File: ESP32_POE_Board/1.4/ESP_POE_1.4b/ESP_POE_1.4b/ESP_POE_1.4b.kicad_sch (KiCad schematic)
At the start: 74 parts, among them J26 USB_C_Receptacle, J5 20021311-00012T4LF, J7 20021311-00012T4LF, Q1 Q12MHz/20pF/10ppm/4P/3.2x2.5mm, Q2 BC817-40(SOT23), Q3 BC817-40(SOT23), SW1 PTS815 SJM 250 SMTR LFS, U1 CH340T(SSOP20W), U3 BL4054B-42TPRN(SOT23-5), U6 ESP32-WROVER-E, U7 SY8089AAAC(SOT23-5), U8 SN74LVC1G04DBVR(SOT23-5)

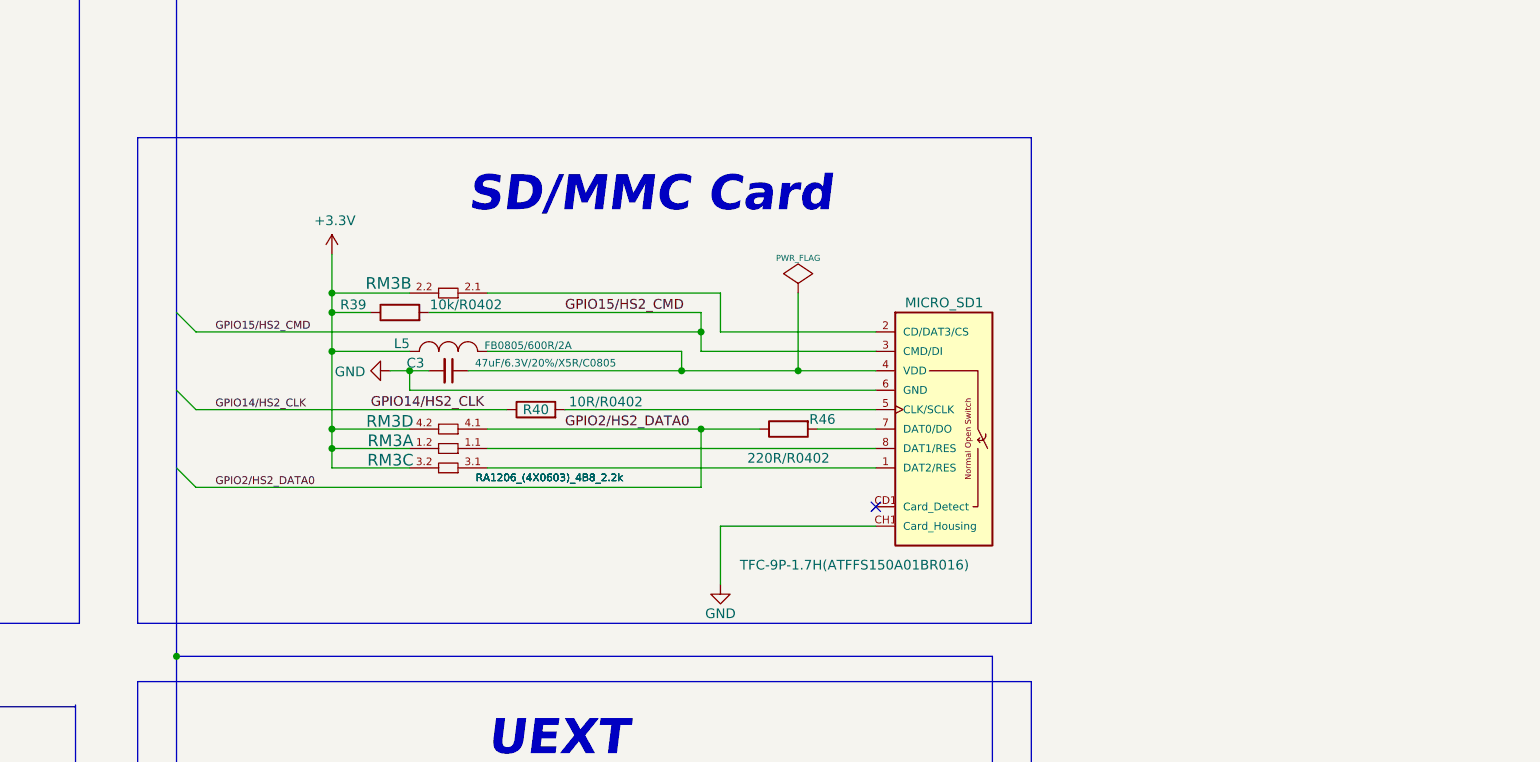
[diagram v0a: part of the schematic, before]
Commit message: fixed 1.4a
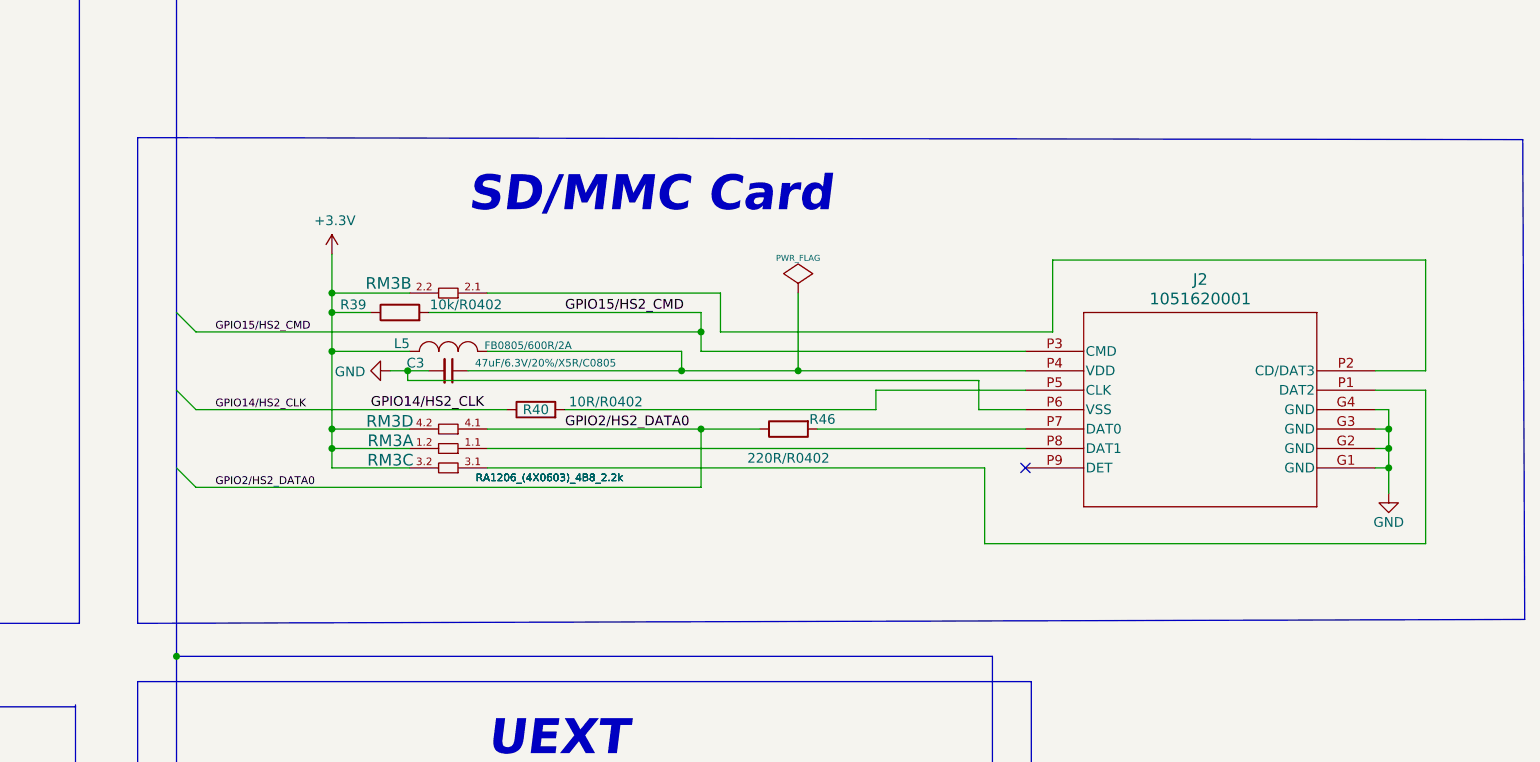
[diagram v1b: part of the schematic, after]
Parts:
- removed MICRO_SD1: TFC-9P-1.7H(ATFFS150A01BR016), OLIMEX_Connectors-FP:uSD(TFC-9P-1.xH(ATFFS150A01BR016)), symbol ESP32-PoE-ISO_Rev_K:MICRO_SD(TFC-9P-1.xH(ATFFS150A01BR016))
- added J2: 1051620001, 105162-0001_MOL, symbol 1051620001:1051620001
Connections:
- net GND: now also J2.G1 (GND), J2.G2 (GND), J2.G3 (GND), J2.G4 (GND), J2.P6 (VSS)
- net GPIO15/HS2_CMD: now also J2.P3 (CMD)
- net at R40.2: now also J2.P5 (CLK)
- net at C3.1, L5.2: now also J2.P4 (VDD)
- net at RM3.2.1: now also J2.P2 (CD/DAT3)
- net at RM3.3.1: now also J2.P1 (DAT2)
- net at RM3.1.1: now also J2.P8 (DAT1)
- net at R46.2: now also J2.P7 (DAT0)
